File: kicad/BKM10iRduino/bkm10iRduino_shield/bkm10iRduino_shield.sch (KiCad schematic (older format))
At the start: 6 parts, among them J1 RJ45, SW1 SW_SPST, U1 TSOP343xx, U2 MAX485E

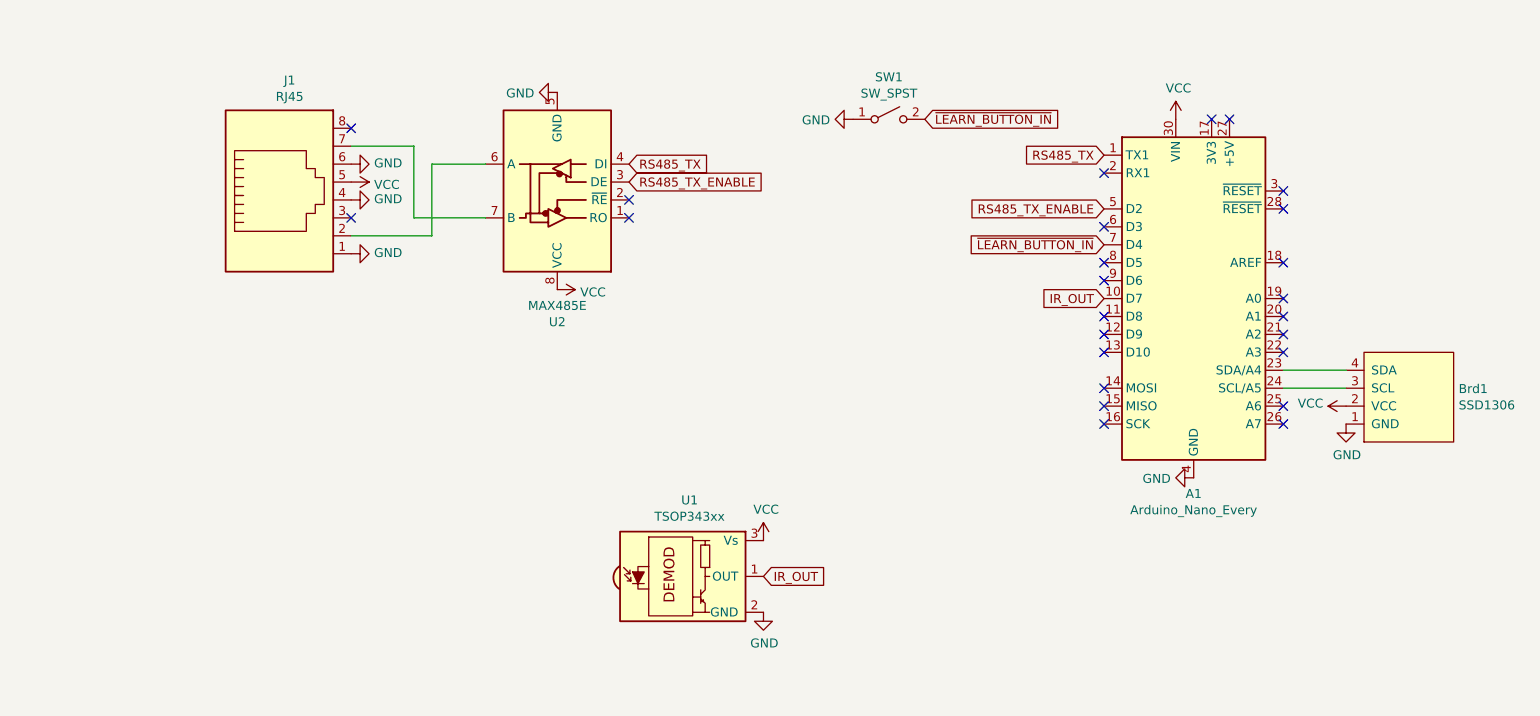
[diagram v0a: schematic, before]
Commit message: updated pcb design
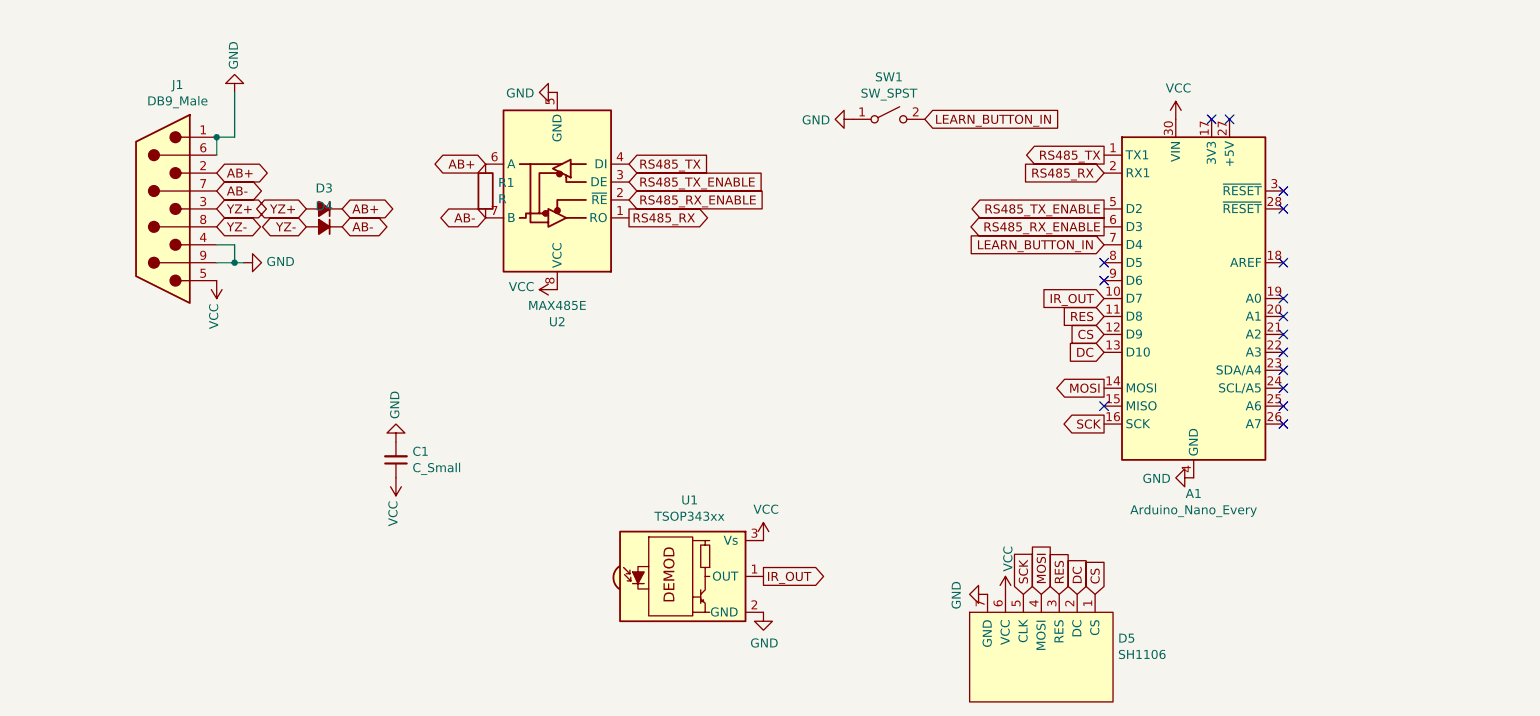
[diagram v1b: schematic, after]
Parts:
- removed Brd1: SSD1306, SSD1306:128x64OLED, symbol SSD1306-128x64_OLED:SSD1306
- removed J1: RJ45, Connector_RJ:RJ45_Amphenol_54602-x08_Horizontal, symbol Connector:RJ45
- added C1: C_Small, Capacitor_SMD:CP_Elec_3x5.3, symbol Device:C_Small
- added D3, D4: D_Small_ALT, Diode_SMD:D_1206_3216Metric_Pad1.42x1.75mm_HandSolder, symbol Device:D_Small_ALT
- added D5: SH1106, Connector_PinHeader_2.54mm:PinHeader_1x07_P2.54mm_Vertical, symbol bkm10:SH1106
- added J1: DB9_Male, Connector_Dsub:DSUB-9_Male_Horizontal_P2.77x2.84mm_EdgePinOffset4.94mm_Housed_MountingHolesOffset7.48mm, symbol Connector:DB9_Male
- added R1: R, Resistor_SMD:R_1206_3216Metric_Pad1.30x1.75mm_HandSolder, symbol Device:R
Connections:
- net GND: now also C1.2, D5.7 (GND), J1.1, J1.4, J1.6, J1.9
- net VCC: now also C1.1, D5.6 (VCC), J1.5
- net RES: now reaches A1.11 (D8)
- net RES: now also D5.3 (RES)
- net CS: now reaches A1.12 (D9)
- net CS: now also D5.1 (CS)
- net DC: now reaches A1.13 (D10)
- net DC: now also D5.2 (DC)
- net MOSI: now reaches A1.14 (MOSI)
- net MOSI: now also D5.4 (MOSI)
- net SCK: now reaches A1.16 (SCK)
- net SCK: now also D5.5 (CLK)
- net RS485_RX: now reaches A1.2 (RX1)
- net RS485_RX: now also U2.1 (RO)
- net RS485_RX_ENABLE: now reaches A1.6 (D3)
- net RS485_RX_ENABLE: now also U2.2 (~RE)
- net AB+: now reaches U2.6 (A)
- net AB+: now also D3.1 (K), J1.2, R1.1
- net AB-: now reaches U2.7 (B)
- net AB-: now also D4.1 (K), J1.7, R1.2
- net ~LEARN_BUTTON_IN renamed LEARN_BUTTON_IN
- new net YZ+: D3.2 (A), J1.3
- new net YZ-: D4.2 (A), J1.8
- no-connect marks 25 -> 16

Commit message: pcb redesign
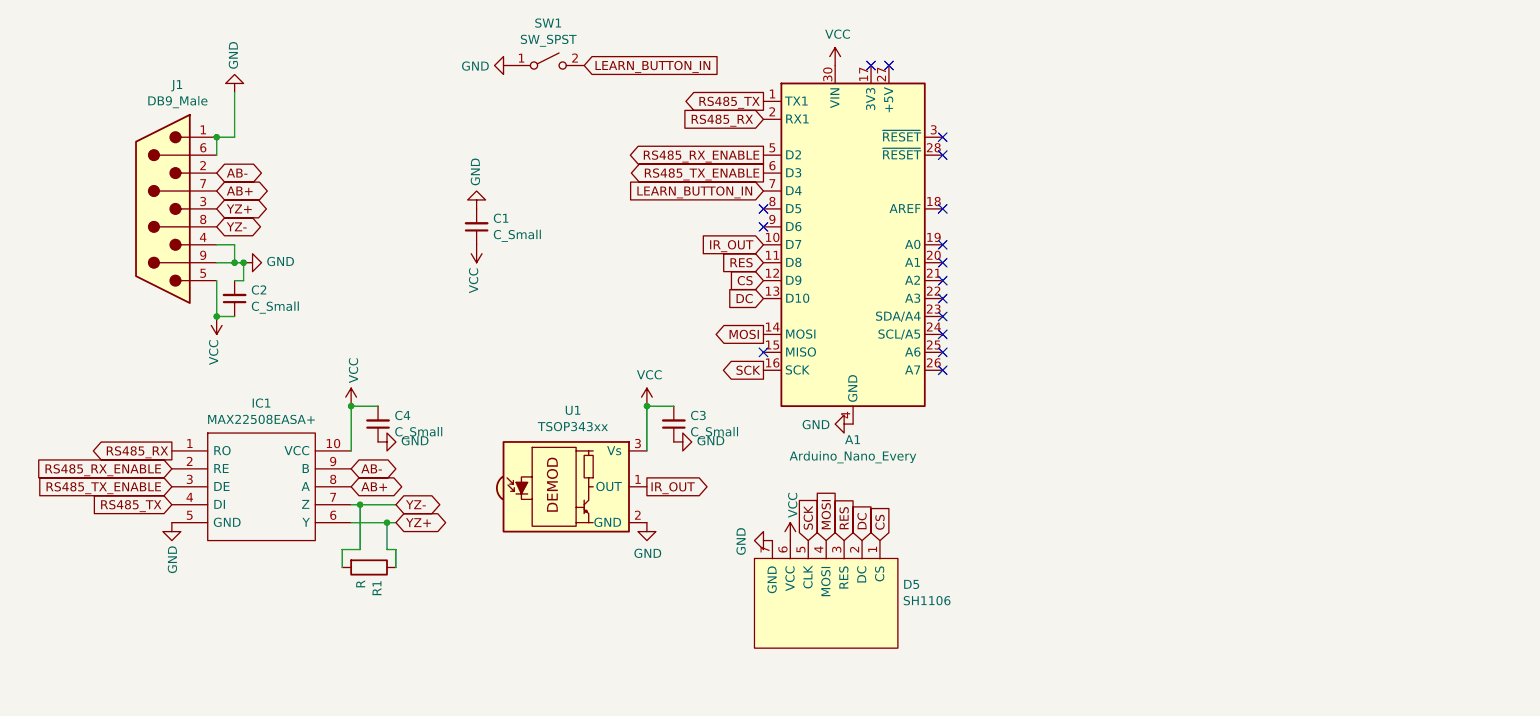
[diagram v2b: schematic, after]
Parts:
- removed D3, D4: D_Small_ALT, Diode_SMD:D_1206_3216Metric_Pad1.42x1.75mm_HandSolder, symbol Device:D_Small_ALT
- removed U2: MAX485E, bkm10rduino:TLL_RS485, symbol Interface_UART:MAX485E
- added C2, C3, C4: C_Small, Capacitor_SMD:C_1812_4532Metric_Pad1.57x3.40mm_HandSolder, symbol Device:C_Small
- added IC1: MAX22508EASA+, SOP50P490X110-10N, symbol SamacSys_Parts:MAX22508EASA+
- C1: footprint Capacitor_SMD:CP_Elec_3x5.3 -> Capacitor_SMD:C_1812_4532Metric_Pad1.57x3.40mm_HandSolder
- J1: footprint Connector_Dsub:DSUB-9_Male_Horizontal_P2.77x2.84mm_EdgePinOffset4.94mm_Housed_MountingHolesOffset7.48mm -> Connector_Dsub:DSUB-9_Male_Vertical_P2.77x2.84mm_MountingHoles
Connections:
- net AB+: now also J1.7, IC1.8 (A); no longer J1.2, R1.1
- net AB-: now also J1.2, IC1.9 (B); no longer J1.7, R1.2
- net GND: now also C2.2, C3.1, C4.1, IC1.5 (GND)
- net RS485_RX: now also IC1.1 (RO)
- net RS485_RX_ENABLE: now also A1.5 (D2), IC1.2 (RE); no longer A1.6 (D3)
- net RS485_TX: now also IC1.4 (DI)
- net RS485_TX_ENABLE: now also A1.6 (D3), IC1.3 (DE); no longer A1.5 (D2)
- net VCC: now also C2.1, C3.2, C4.2, IC1.10 (VCC)
- net YZ+: now also R1.1, IC1.6 (Y)
- net YZ-: now also R1.2, IC1.7 (Z)
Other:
- moved on the sheet: A1, C1, D5, R1, SW1, U1
